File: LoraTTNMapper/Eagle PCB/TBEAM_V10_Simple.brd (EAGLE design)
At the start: 100 x 80 mm, 19 parts, among them IC2 ULN2003AD

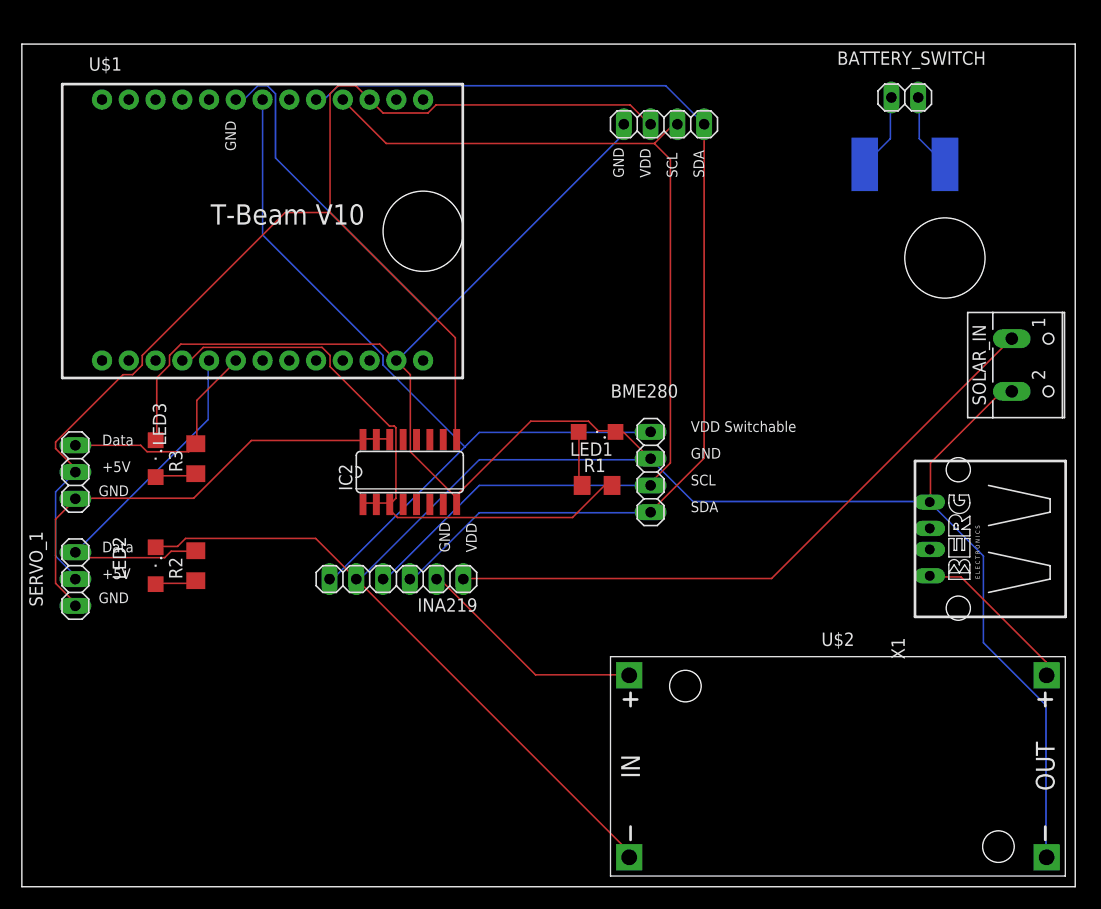
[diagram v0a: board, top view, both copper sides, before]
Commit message: PCB
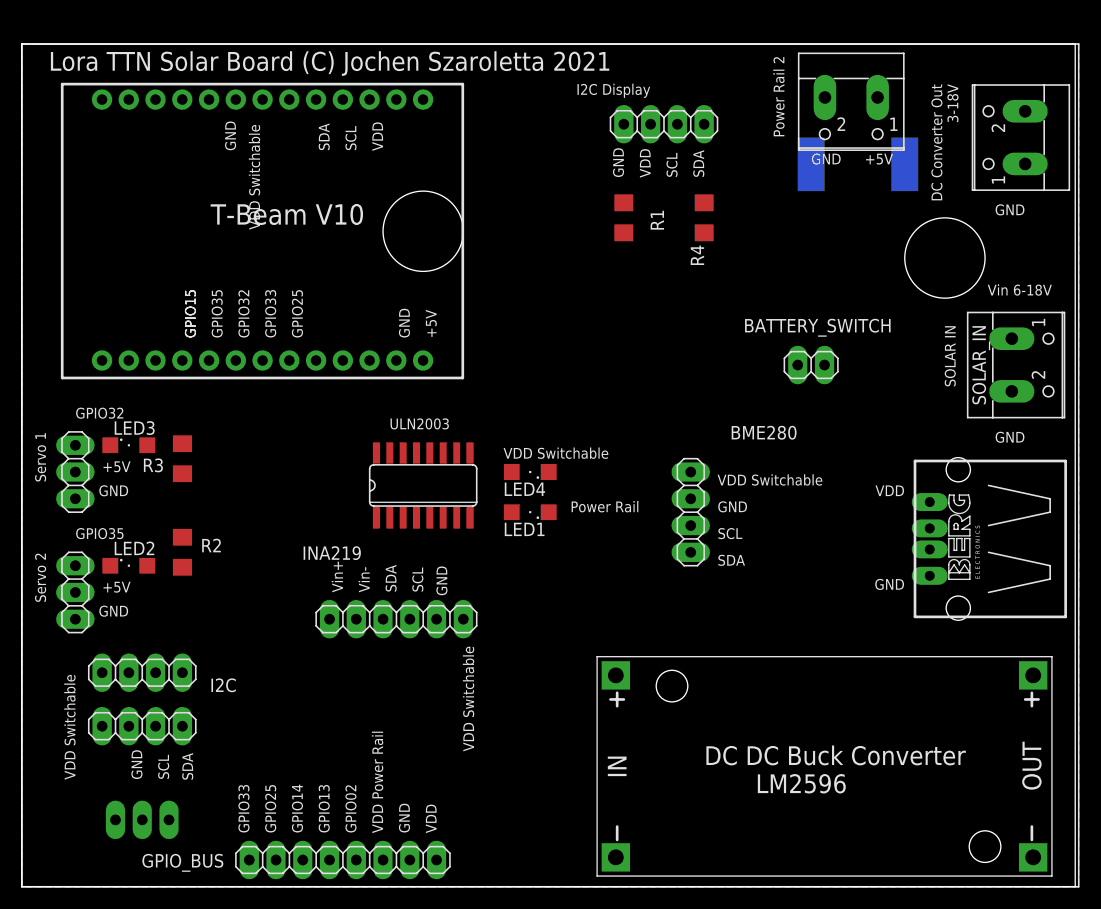
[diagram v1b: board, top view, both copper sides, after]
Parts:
- added GPIO04: FAST LED, pinhead:1X03
- added GPIO_BUS: (no value), pinhead:1X08
- added I2C, I2C1: (no value), pinhead:1X04
- added LED4: VDD Switchable, led:SML1206
- added POWER_RAIL2, V5: (no value), con-wago-500:W237-102
- added R4: 220, resistor:R1206
- LED2: value (none) -> GPIO35
- LED3: value (none) -> GPIO32
- R1, R2, R3: value (none) -> 220
- moved BATTERY_SWITCH 26.9 mm to (74.9, 49.5)
- moved R1 25.5 mm to (57.1, 63.5), turned to 90 degrees
- moved LED1 9.92 mm to (48.3, 35.6)
- moved BME280 5.39 mm to (63.5, 35.6)
- moved BAT_IN 5.08 mm to (74.9, 68.6)
- moved BAT_OUT 3.81 mm to (83.8, 68.6)
- moved INA219 3.81 mm to (35.6, 25.4), turned to 0 degrees
- moved LED3 2.84 mm to (10.2, 41.9), turned to 0 degrees
- moved LED2 2.54 mm to (10.2, 30.5), turned to 0 degrees
- moved R2 1.80 mm to (15.2, 31.8)
- moved IC2 1.80 mm to (38.1, 38.1)
- moved R3 1.27 mm to (15.2, 40.6), turned to 270 degrees
- moved SERVO_1 1.27 mm to (5.08, 27.9)
- moved U$2 1.27 mm to (76.2, 11.4)
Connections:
- removed net POWER_RAIL_1_VDD: IC2.14, IC2.15, IC2.16, SERVO_1.1, SERVO_2/GPIO32.1
- new net GPIO02: GPIO_BUS.5, U$1.11
- new net GPIO04: GPIO04.1, U$1.23
- new net GPIO13: GPIO_BUS.4, U$1.10
- new net GPIO14: GPIO_BUS.3, U$1.9
- new net GPIO25: GPIO_BUS.2, U$1.8
- new net GPIO33: GPIO_BUS.1, U$1.7
- new net GPIO36: IC2.4, IC2.5, IC2.6, IC2.7, U$1.1
- new net N$11: LED4.A, R4.1
- new net N$12: IC2.10, IC2.11, IC2.12, IC2.13, POWER_RAIL2.2
- new net POWER_RAIL_1_GND: GPIO_BUS.6, IC2.14, IC2.15, IC2.16, SERVO_1.1, SERVO_2/GPIO32.1
- net +5V: now also GPIO04.2, IC2.9, POWER_RAIL2.1, SERVO_1.2, SERVO_2/GPIO32.2
- net GND: now also GPIO04.3, GPIO_BUS.7, I2C.3, I2C1.3, LED4.C, V5.1
- net N$8: now also V5.2
- net SCL: now also I2C.2, I2C1.2, U$1.18; no longer U$1.17
- net SDA: now also I2C.1, I2C1.1, U$1.17; no longer U$1.18
- net VDD: now also GPIO_BUS.8; no longer IC2.9, SERVO_1.2, SERVO_2/GPIO32.2
- net VDD_SWITCHABLE: now also I2C.4, I2C1.4, R4.2
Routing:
- net GND: track 306.5 -> 0.00 mm
- net VDD: track 121.7 -> 0.00 mm
- net SDA: track 103.3 -> 0.00 mm
- net SCL: track 97.3 -> 0.00 mm
- net VDD_SWITCHABLE: track 77.2 -> 0.00 mm
- net V_IN_+: track 61.5 -> 0.00 mm
- net GPIO15: track 58.2 -> 0.00 mm
- net POWER_RAIL_1_VDD: track 44.1 -> 0.00 mm
- net GPIO35: track 35.4 -> 0.00 mm
- net V_OUT_+: track 22.1 -> 0.00 mm
- net GPIO32: track 21.6 -> 0.00 mm
- net N$8: track 15.7 -> 0.00 mm
- net N$9: track 7.40 -> 0.00 mm
- net N$10: track 7.40 -> 0.00 mm
- net N$4: track 5.21 -> 0.00 mm
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- added copper zone on layer 1, net GND
- added copper zone on layer 16, net GND
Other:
- board text added: "+5v"
- board text added: "---------------------------------- GPIO 04 = FAST Led GPIO 15 = Power Rail 1 GPIO 35 = Servo 1 GPIO 32 = Servo 2 GPIO 36 = Power Rail 2 ---------------------------------"
- board text added: "DC Converter Out 3-18V"
- board text added: "DC DC Buck Converter LM2596"
- board text added: "GPIO02"
- board text added: "GPIO04"
- board text added: "GPIO13"
- board text added: "GPIO14"
- board text added: "GPIO15"
- board text added: "GPIO25"
- board text added: "GPIO32"
- board text added: "GPIO33"
- board text added: "GPIO35"
- board text added: "Lora TTN Solar Board (C) Jochen Szaroletta 2021"
- board text added: "Power Rail"
- board text added: "Power Rail 2"
- board text added: "SOLAR IN"
- board text added: "Servo 1"
- board text added: "Servo 2"
- board text added: "ULN2003"
- board text added: "VDD Power Rail"
- board text added: "Vin 6-18V"
- board text added: "Vin+"
- board text added: "Vin-"
- board text added: "https://github.com/MrFlexi/LoraTTNMapper"
- board text removed: "+18V"
- board text removed: "Data"
